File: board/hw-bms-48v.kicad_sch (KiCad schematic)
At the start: 41 parts, among them J1 BATT, J2 PROG, J3 CURRENT, J4 TEMP, J5 ILI9225, U1 BD9G341EFJ, U2 ESP32-C3-WROOM-02, U2 LM1117MP-3.3

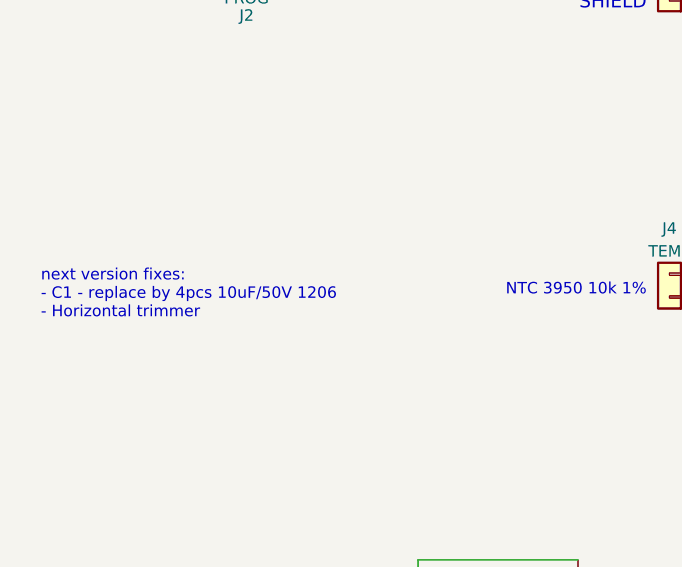
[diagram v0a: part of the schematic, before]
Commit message: WIP
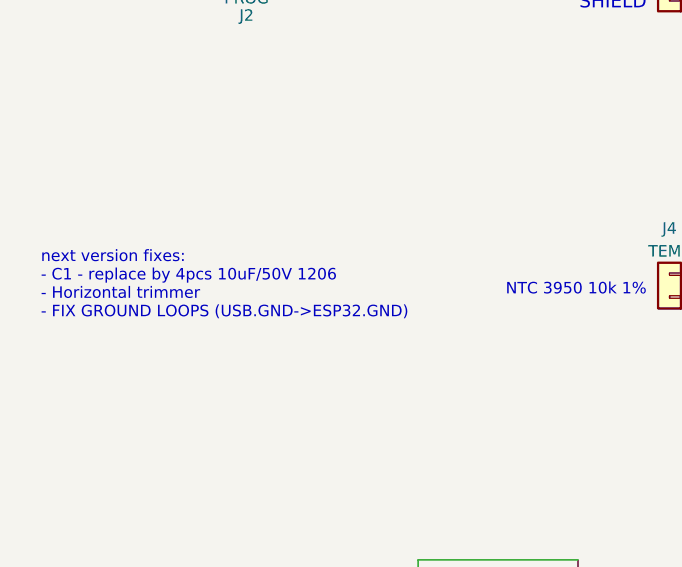
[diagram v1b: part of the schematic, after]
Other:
- note added: "next version fixes: - C1 - replace by 4pcs 10uF/50V 1206 - Horizontal trimmer - FIX GROUND LOOPS (USB.GND->ESP32.GND)"
- note removed: "next version fixes: - C1 - replace by 4pcs 10uF/50V 1206 - Horizontal trimmer"
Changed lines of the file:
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@@
     (stroke (width 0) (type default))
   )
-  (text "next version fixes:\n- C1 - replace by 4pcs 10uF/50V 1206\n- Horizontal trimmer" (exclude_from_sim no)
+  (text "next version fixes:\n- C1 - replace by 4pcs 10uF/50V 1206\n- Horizontal trimmer\n- FIX GROUND LOOPS (USB.GND->ESP32.GND)" (exclude_from_sim no)
     (at 26.67 109.22 0)
     (effects (font (size 1.27 1.27)) (justify left bottom))

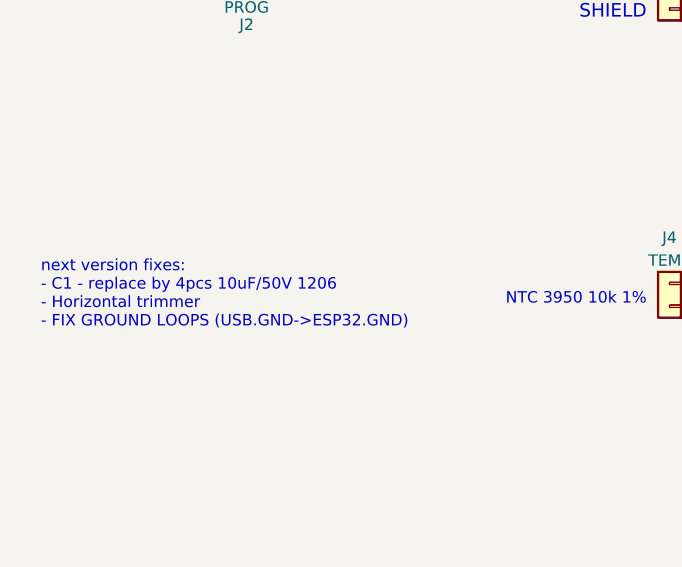
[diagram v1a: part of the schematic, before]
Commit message: WIP
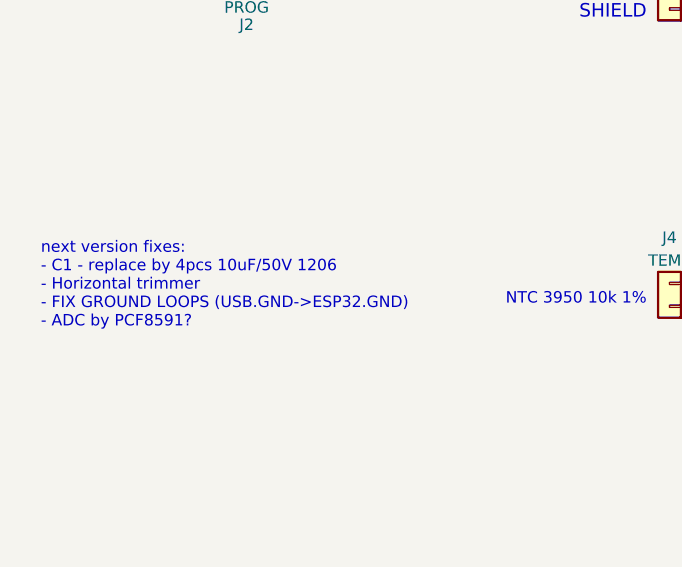
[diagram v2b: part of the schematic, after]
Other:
- note added: "next version fixes: - C1 - replace by 4pcs 10uF/50V 1206 - Horizontal trimmer - FIX GROUND LOOPS (USB.GND->ESP32.GND) - ADC by PCF8591?"
- note removed: "next version fixes: - C1 - replace by 4pcs 10uF/50V 1206 - Horizontal trimmer - FIX GROUND LOOPS (USB.GND->ESP32.GND)"
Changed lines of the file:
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@@
     (stroke (width 0) (type default))
   )
-  (text "next version fixes:\n- C1 - replace by 4pcs 10uF/50V 1206\n- Horizontal trimmer\n- FIX GROUND LOOPS (USB.GND->ESP32.GND)" (exclude_from_sim no)
+  (text "next version fixes:\n- C1 - replace by 4pcs 10uF/50V 1206\n- Horizontal trimmer\n- FIX GROUND LOOPS (USB.GND->ESP32.GND)\n- ADC by PCF8591?" (exclude_from_sim no)
     (at 26.67 109.22 0)
     (effects (font (size 1.27 1.27)) (justify left bottom))
